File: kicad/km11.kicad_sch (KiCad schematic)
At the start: 8 parts, among them J1 DEC-FLIP-CHIP_CONN-DEC-DOUBLE, U1 ATtiny1616-S, U2 PCF8574T, U3 PCF8574T, U4 PCF8574T, U5 PCF8574T, U6 PCF8574T, U7 PCF8574T

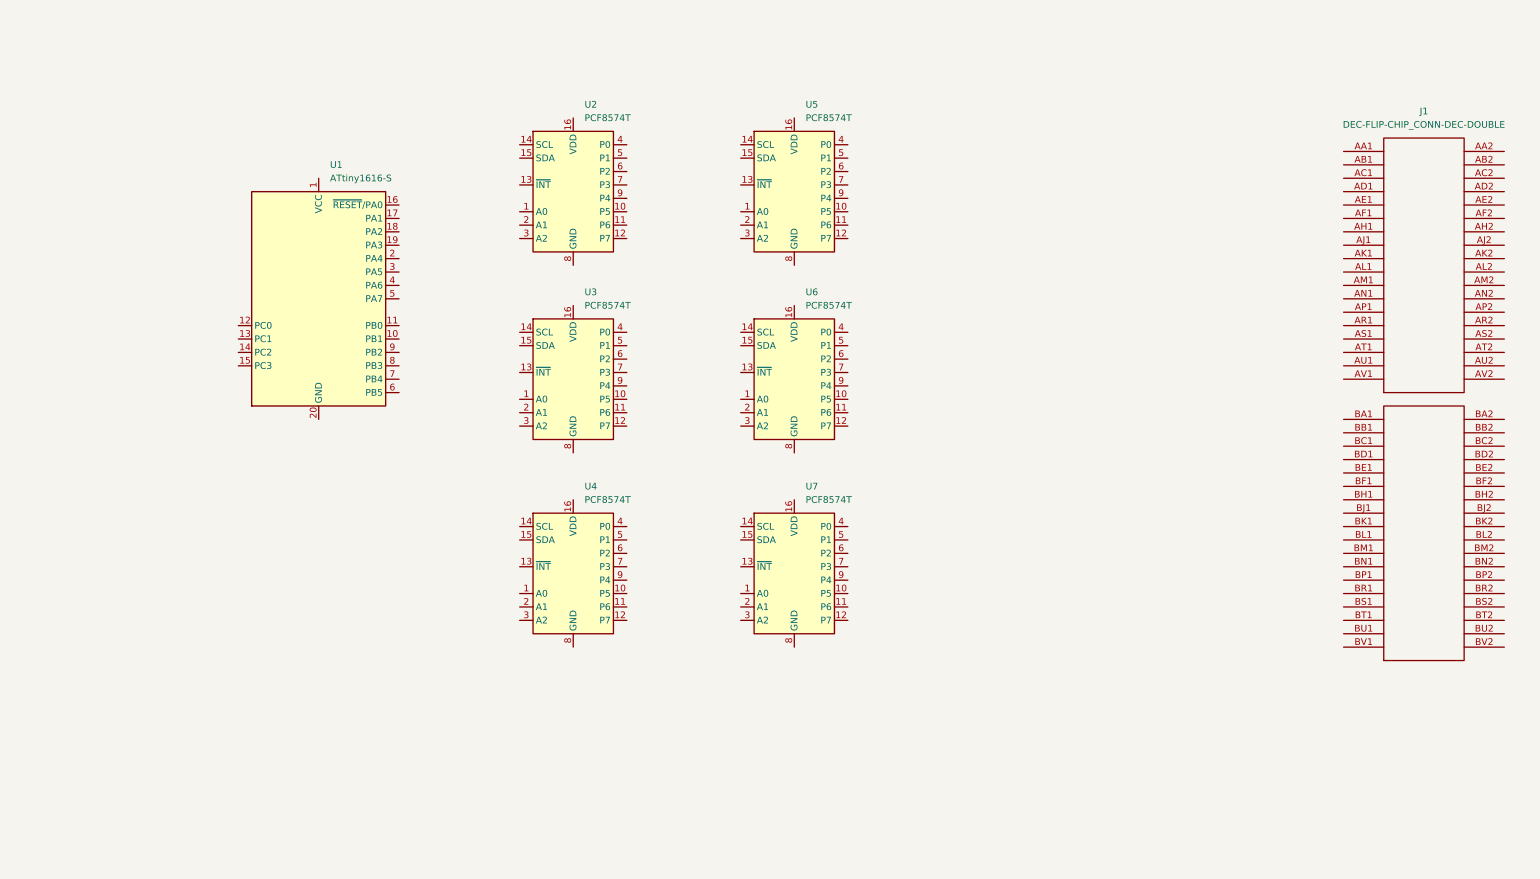
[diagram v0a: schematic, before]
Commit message: First small parts
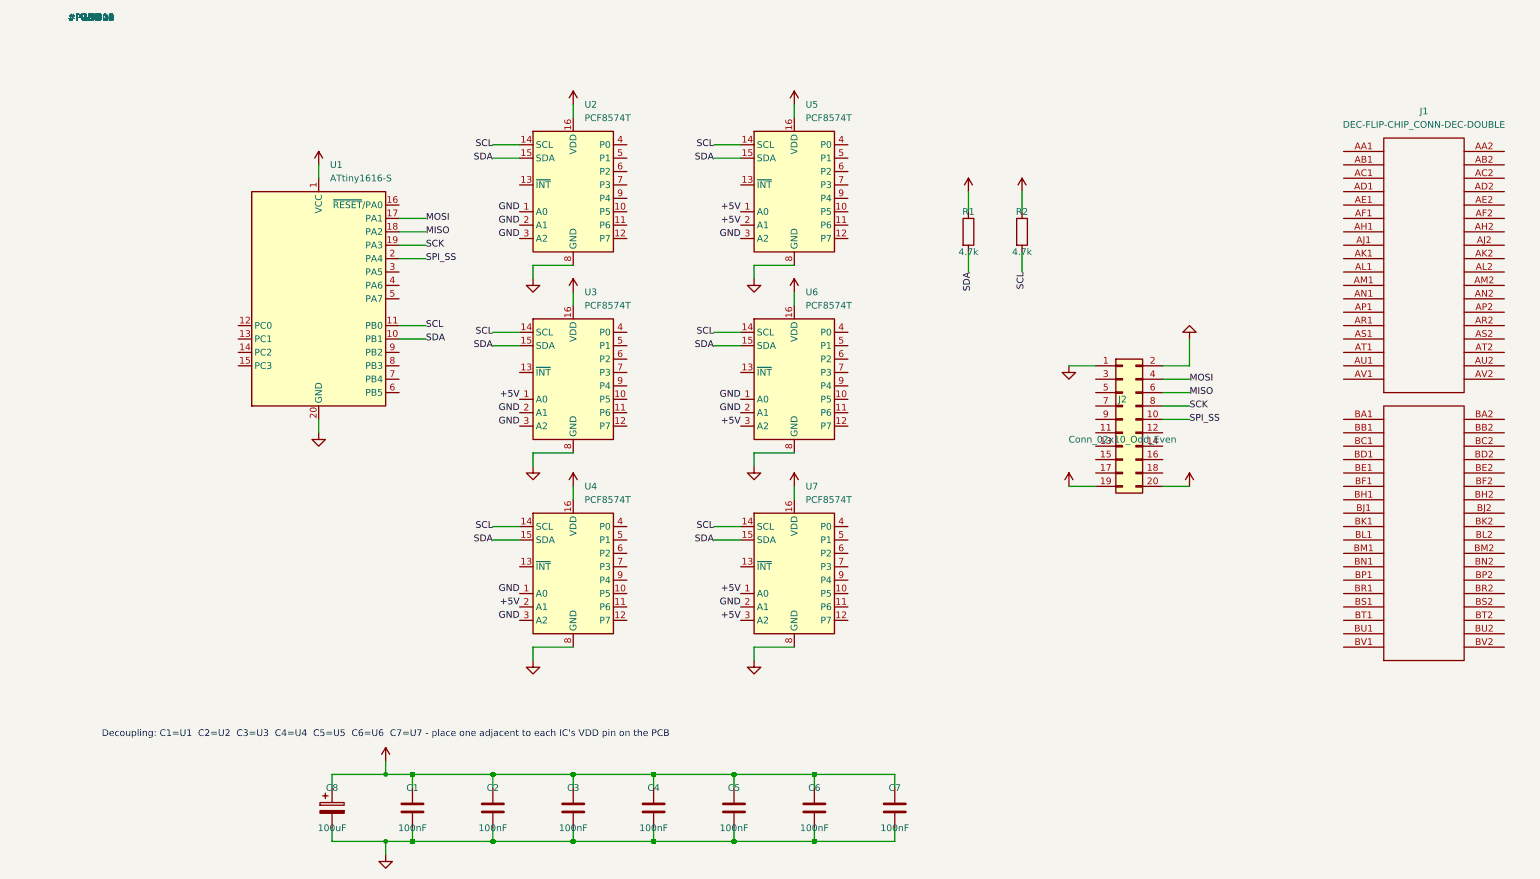
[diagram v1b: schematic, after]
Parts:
- added C1, C2, C3, C4, C5, C6, C7: 100nF, Capacitor_SMD:C_0805_2012Metric, symbol Device:C
- added C8: 100uF, Capacitor_SMD:CP_Elec_6.3x7.7, symbol Device:C_Polarized
- added J2: Conn_02x10_Odd_Even, Connector_PinHeader_2.54mm:PinHeader_2x10_P2.54mm_Vertical, symbol Connector_Generic:Conn_02x10_Odd_Even
- added R1, R2: 4.7k, Resistor_SMD:R_0805_2012Metric, symbol Device:R
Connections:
- net GND: now reaches U4.1 (A0)
- net GND: now also U1.20 (GND), U2.1 (A0), U2.2 (A1), U2.3 (A2), U2.8 (GND), U3.2 (A1), U3.3 (A2), U3.8 (GND), U4.3 (A2), U4.8 (GND), U5.3 (A2), U5.8 (GND), U6.1 (A0), U6.2 (A1), U6.8 (GND), U7.2 (A1), U7.8 (GND), C1.2, C2.2, C3.2, C4.2, C5.2, C6.2, C7.2, C8.2, J2.1 (Pin_1), J2.2 (Pin_2)
- net SCL: now reaches U4.14 (SCL)
- net SCL: now also U1.11 (PB0), U2.14 (SCL), U3.14 (SCL), U5.14 (SCL), U6.14 (SCL), U7.14 (SCL), R2.2
- net SDA: now reaches U4.15 (SDA)
- net SDA: now also U1.10 (PB1), U2.15 (SDA), U3.15 (SDA), U5.15 (SDA), U6.15 (SDA), U7.15 (SDA), R1.2
- net +5V: now reaches U4.16 (VDD)
- net +5V: now also U1.1 (VCC), U2.16 (VDD), U3.1 (A0), U3.16 (VDD), U4.2 (A1), U5.1 (A0), U5.16 (VDD), U5.2 (A1), U6.16 (VDD), U6.3 (A2), U7.1 (A0), U7.16 (VDD), U7.3 (A2), C1.1, C2.1, C3.1, C4.1, C5.1, C6.1, C7.1, C8.1, J2.19 (Pin_19), J2.20 (Pin_20), R1.1, R2.1
- net MOSI: now reaches U1.17 (PA1)
- net MOSI: now also J2.4 (Pin_4)
- net MISO: now reaches U1.18 (PA2)
- net MISO: now also J2.6 (Pin_6)
- net SCK: now reaches U1.19 (PA3)
- net SCK: now also J2.8 (Pin_8)
- net SPI_SS: now reaches U1.2 (PA4)
- net SPI_SS: now also J2.10 (Pin_10)
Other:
- note added: "Decoupling: C1=U1 C2=U2 C3=U3 C4=U4 C5=U5 C6=U6 C7=U7 - place one adjacent to each IC's VDD pin on the PCB"
